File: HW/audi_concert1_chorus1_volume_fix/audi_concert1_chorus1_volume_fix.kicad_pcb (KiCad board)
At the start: 2 copper layers, 32.8 x 26.2 mm, 40 parts, among them CON1 I2C_to_TDA, CON2 USB, CON3 SPI_TO_PANEL, CON4 JLINK, U1 68HC05_PLCC, U2 AP1117-33, U3 STM32F103C8Tx, U4 MAX809, Y1 32.768kHz, Y2 8MHz

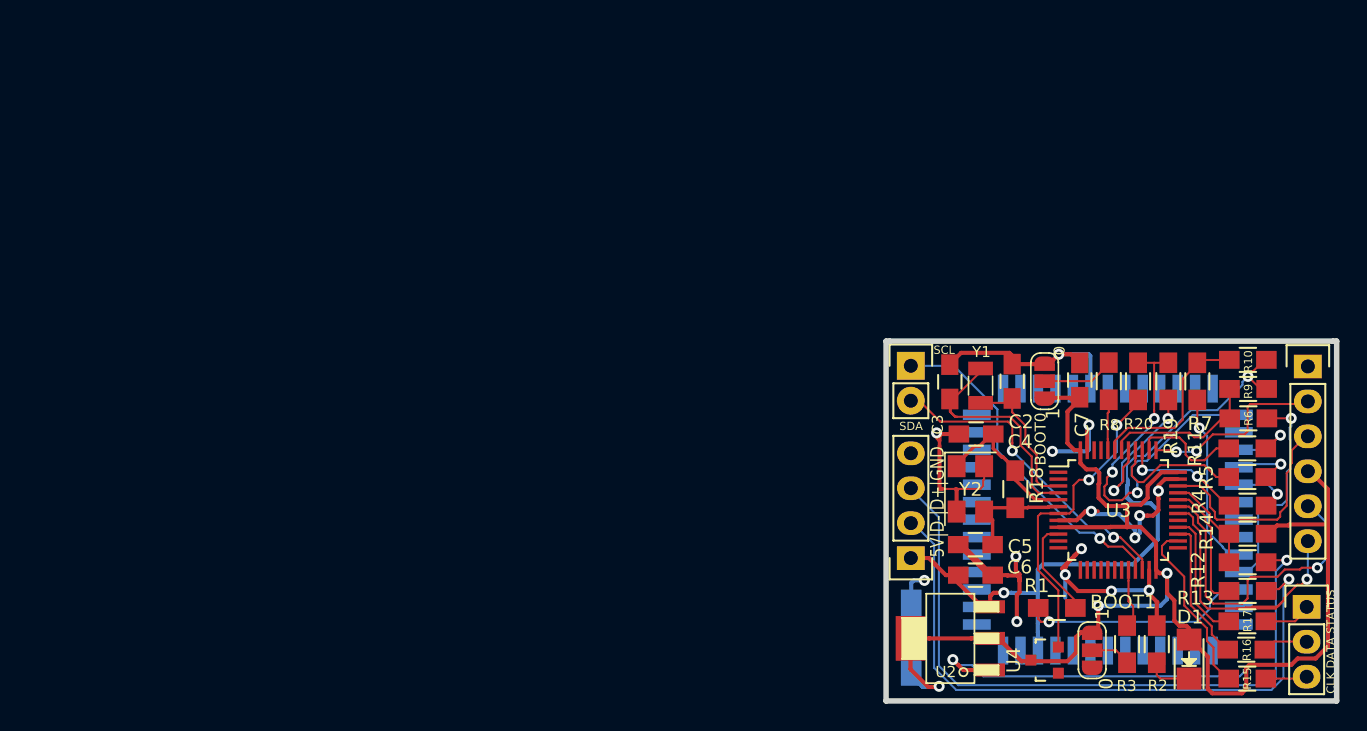
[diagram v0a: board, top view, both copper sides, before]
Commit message: pcb update
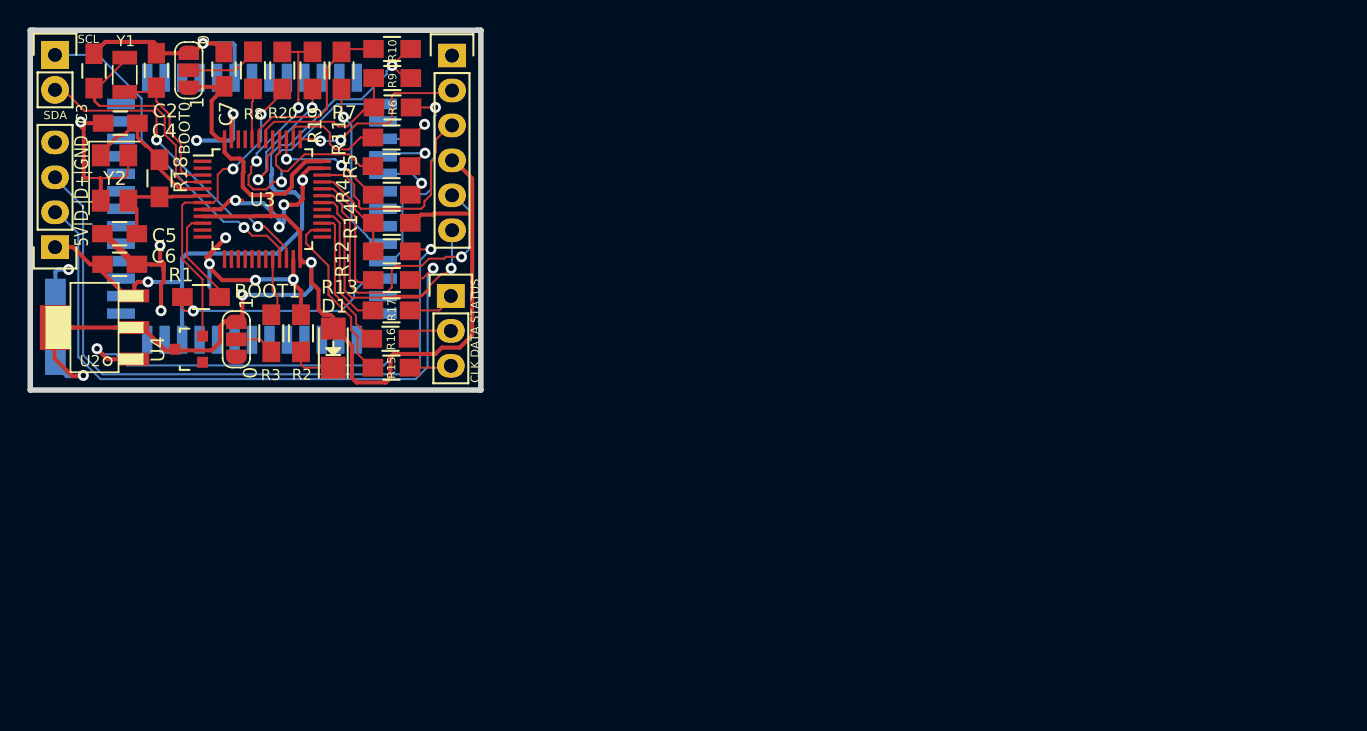
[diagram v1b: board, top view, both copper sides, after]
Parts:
- moved C8 66.2 mm to (103.4, 92.7)
- moved CON1 66.2 mm to (103.4, 72.9)
- moved Y1 66.2 mm to (108.5, 74.4)
- moved BOOT0 66.2 mm to (113.1, 74.0)
- moved BOOT1 66.2 mm to (116.6, 93.6)
- moved C2 66.2 mm to (110.8, 74.0)
- moved C4 66.2 mm to (108.1, 77.9)
- moved C5 66.2 mm to (108.1, 85.9)
- moved C6 66.2 mm to (108.1, 88.1)
- moved C7 66.2 mm to (115.7, 73.9)
- moved R1 66.2 mm to (114.0, 90.5)
- moved R11 66.2 mm to (127.9, 78.9)
- moved R13 66.2 mm to (127.9, 89.3)
- moved R15 66.2 mm to (127.9, 95.7)
- moved R18 66.2 mm to (111.0, 81.9)
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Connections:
- BOOT0 pad 1: GND -> (no net)
- BOOT0 pad 2: /BOOT0 -> (no net)
- BOOT0 pad 3: 3V3 -> (no net)
- BOOT1 pad 1: GND -> (no net)
- BOOT1 pad 2: /BOOT1 -> (no net)
- BOOT1 pad 3: 3V3 -> (no net)
- C2 pad 1: /OSC32IN -> (no net)
- C2 pad 2: GND -> (no net)
- C3 pad 1: GND -> (no net)
- C3 pad 2: /OSC32OUT -> (no net)
- C4 pad 1: /OSCIN -> (no net)
- C4 pad 2: GND -> (no net)
- C5 pad 1: GND -> (no net)
- C5 pad 2: /OSCOUT -> (no net)
- C6 pad 1: 5V -> (no net)
- C6 pad 2: GND -> (no net)
- C7 pad 1: 3V3 -> (no net)
- C7 pad 2: GND -> (no net)
- C8 pad 1: 3V3 -> (no net)
- C8 pad 2: GND -> (no net)
- CON1 pad 1: /SCL_TO_TDA -> (no net)
- CON1 pad 2: /SDA_TO_TDA -> (no net)
- CON2 pad 1: 5V -> (no net)
- CON2 pad 2: Net-(CON2-Pad2) -> (no net)
- CON2 pad 3: Net-(CON2-Pad3) -> (no net)
- CON2 pad 4: GND -> (no net)
- CON3 pad 1: /STATUS_TO_PANEL -> (no net)
- CON3 pad 2: /DATA_TO_PANEL -> (no net)
- CON3 pad 3: /CLOCK_TO_PANEL -> (no net)
- CON4 pad 1: GND -> (no net)
- CON4 pad 2: /SWDCLK -> (no net)
- CON4 pad 3: /SWDIO -> (no net)
- CON4 pad 4: 3V3 -> (no net)
- CON4 pad 5: /RX -> (no net)
- CON4 pad 6: /TX -> (no net)
- D1 pad 1: Net-(D1-Pad1) -> (no net)
- D1 pad 2: 3V3 -> (no net)
- R1 pad 1: /GALA -> (no net)
- R1 pad 2: Net-(R1-Pad2) -> (no net)
- R10 pad 1: Net-(R10-Pad1) -> (no net)
- R10 pad 2: 5V -> (no net)
- R11 pad 1: Net-(R11-Pad1) -> (no net)
- R11 pad 2: /STATUS_FROM_MCU -> (no net)
- R12 pad 1: /USB+ -> (no net)
- R12 pad 2: Net-(CON2-Pad3) -> (no net)
- R13 pad 1: Net-(CON2-Pad2) -> (no net)
- R13 pad 2: /USB- -> (no net)
- R14 pad 1: 3V3 -> (no net)
- R14 pad 2: /USB+ -> (no net)
- R15 pad 1: /CLOCK_TO_PANEL -> (no net)
- R15 pad 2: Net-(R15-Pad2) -> (no net)
- R16 pad 1: /DATA_TO_PANEL -> (no net)
- R16 pad 2: Net-(R16-Pad2) -> (no net)
- R17 pad 1: /STATUS_TO_PANEL -> (no net)
- R17 pad 2: Net-(R17-Pad2) -> (no net)
- R18 pad 1: /OSCOUT -> (no net)
- R18 pad 2: /OSCIN -> (no net)
- R19 pad 1: /RESET_KA -> (no net)
- R19 pad 2: Net-(R19-Pad2) -> (no net)
- R2 pad 1: GND -> (no net)
- R2 pad 2: Net-(D1-Pad1) -> (no net)
- R20 pad 1: /RESET_KA -> (no net)
- R20 pad 2: /RESET -> (no net)
- R3 pad 1: Net-(R3-Pad1) -> (no net)
- R3 pad 2: /BOOT1 -> (no net)
- R4 pad 1: Net-(R4-Pad1) -> (no net)
- R4 pad 2: /CLOCK_FROM_MCU -> (no net)
- R5 pad 1: /DATA_FROM_MCU -> (no net)
- R5 pad 2: Net-(R5-Pad2) -> (no net)
- R6 pad 1: Net-(R6-Pad1) -> (no net)
- R6 pad 2: /SCL_FROM_MOTO -> (no net)
- R7 pad 1: Net-(R10-Pad1) -> (no net)
- R7 pad 2: /SDA_FROM_MOTO -> (no net)
- R8 pad 1: Net-(R8-Pad1) -> (no net)
- R8 pad 2: /BOOT0 -> (no net)
- R9 pad 1: 5V -> (no net)
- R9 pad 2: Net-(R6-Pad1) -> (no net)
- U1 pad 10: 5V -> (no net)
- U1 pad 23: /GALA -> (no net)
- U1 pad 24: /SCL_FROM_MOTO -> (no net)
- U1 pad 25: /SDA_FROM_MOTO -> (no net)
- U1 pad 29: /CLOCK_FROM_MCU -> (no net)
- U1 pad 30: /DATA_FROM_MCU -> (no net)
- U1 pad 31: /STATUS_FROM_MCU -> (no net)
- U1 pad 33: /RESET_KA -> (no net)
- U1 pad 41: GND -> (no net)
- U2 pad 1: GND -> (no net)
- U2 pad 2: 3V3 -> (no net)
- U2 pad 3: 5V -> (no net)
- U3 pad 10: Net-(R1-Pad2) -> (no net)
- U3 pad 20: Net-(R3-Pad1) -> (no net)
- U3 pad 21: /SCL_TO_TDA -> (no net)
- U3 pad 22: /SDA_TO_TDA -> (no net)
- U3 pad 23: GND -> (no net)
- U3 pad 24: 3V3 -> (no net)
- U3 pad 26: Net-(R15-Pad2) -> (no net)
- U3 pad 27: Net-(R16-Pad2) -> (no net)
- U3 pad 28: Net-(R17-Pad2) -> (no net)
- U3 pad 3: /OSC32IN -> (no net)
- U3 pad 30: /TX -> (no net)
- U3 pad 31: /RX -> (no net)
- U3 pad 32: /USB- -> (no net)
- U3 pad 33: /USB+ -> (no net)
- U3 pad 34: /SWDIO -> (no net)
- U3 pad 35: GND -> (no net)
- U3 pad 36: 3V3 -> (no net)
- U3 pad 37: /SWDCLK -> (no net)
- U3 pad 38: Net-(R11-Pad1) -> (no net)
- U3 pad 39: Net-(R4-Pad1) -> (no net)
- U3 pad 4: /OSC32OUT -> (no net)
- U3 pad 40: Net-(R5-Pad2) -> (no net)
- U3 pad 41: Net-(R19-Pad2) -> (no net)
- U3 pad 42: Net-(R6-Pad1) -> (no net)
- U3 pad 43: Net-(R10-Pad1) -> (no net)
- U3 pad 44: Net-(R8-Pad1) -> (no net)
- U3 pad 47: GND -> (no net)
- U3 pad 48: 3V3 -> (no net)
- U3 pad 5: /OSCIN -> (no net)
- U3 pad 6: /OSCOUT -> (no net)
- U3 pad 7: /RESET -> (no net)
- U3 pad 8: GND -> (no net)
- U3 pad 9: 3V3 -> (no net)
- U4 pad 1: GND -> (no net)
- U4 pad 2: /RESET -> (no net)
- U4 pad 3: 3V3 -> (no net)
- Y1 pad 1: /OSC32IN -> (no net)
- Y1 pad 2: /OSC32OUT -> (no net)
- Y2 pad 1: /OSCIN -> (no net)
- Y2 pad 2: GND -> (no net)
- Y2 pad 3: /OSCOUT -> (no net)
- Y2 pad 4: GND -> (no net)
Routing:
- net (no net): track 0.00 -> 796.3 mm, vias 0 -> 45
- net GND: track 106.9 -> 0.00 mm, vias 16 -> 0
- net 3V3: track 103.2 -> 0.00 mm, vias 3 -> 0
- net 5V: track 52.3 -> 0.00 mm, vias 2 -> 0
- net Net-(CON2-Pad3): track 49.5 -> 0.00 mm, vias 1 -> 0
- net Net-(CON2-Pad2): track 47.2 -> 0.00 mm, vias 1 -> 0
- net /RESET_KA: track 27.5 -> 0.00 mm, vias 3 -> 0
- net /SCL_TO_TDA: track 25.4 -> 0.00 mm, vias 1 -> 0
- net /TX: track 23.5 -> 0.00 mm, vias 1 -> 0
- net /RX: track 23.5 -> 0.00 mm, vias 1 -> 0
- net /SDA_TO_TDA: track 23.4 -> 0.00 mm, vias 2 -> 0
- net /RESET: track 23.2 -> 0.00 mm, vias 2 -> 0
- net /OSC32OUT: track 18.1 -> 0.00 mm
- net /GALA: track 16.7 -> 0.00 mm, vias 1 -> 0
- net /SWDIO: track 16.0 -> 0.00 mm
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- added copper zone on B.Cu, net (none)
- added copper zone on F.Cu, net (none)
- removed copper zone on B.Cu, net GND
- removed copper zone on F.Cu, net GND
